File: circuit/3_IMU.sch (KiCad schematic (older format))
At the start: 23 parts

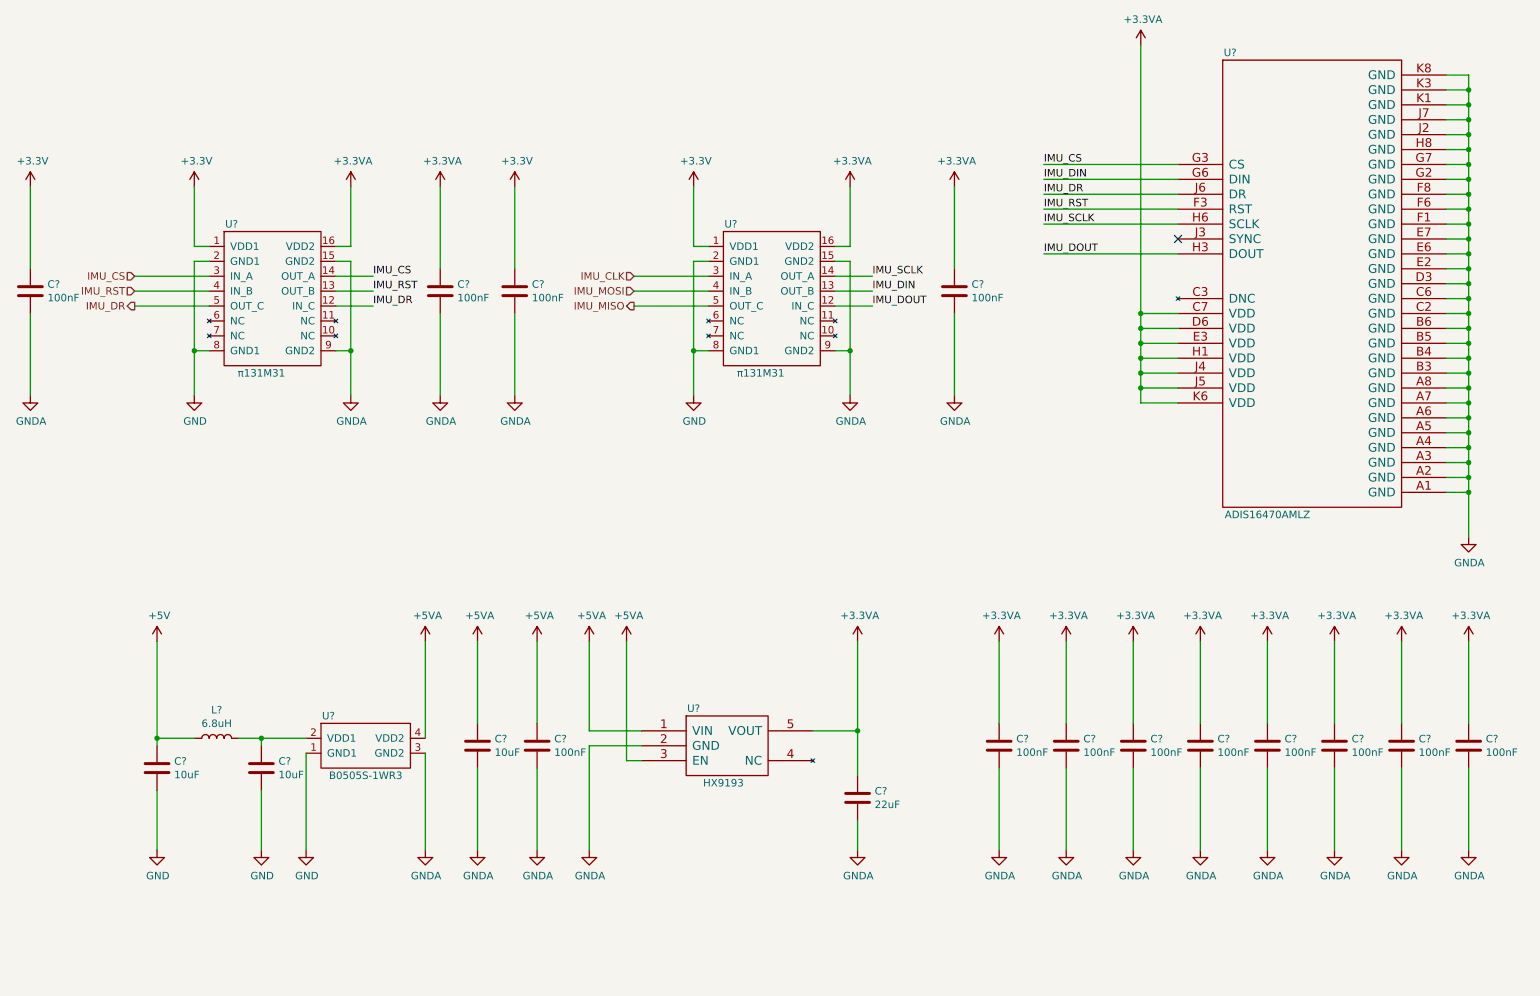
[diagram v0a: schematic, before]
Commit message: Adjust the schematic layout and add annotations to make the schematic more beautiful.
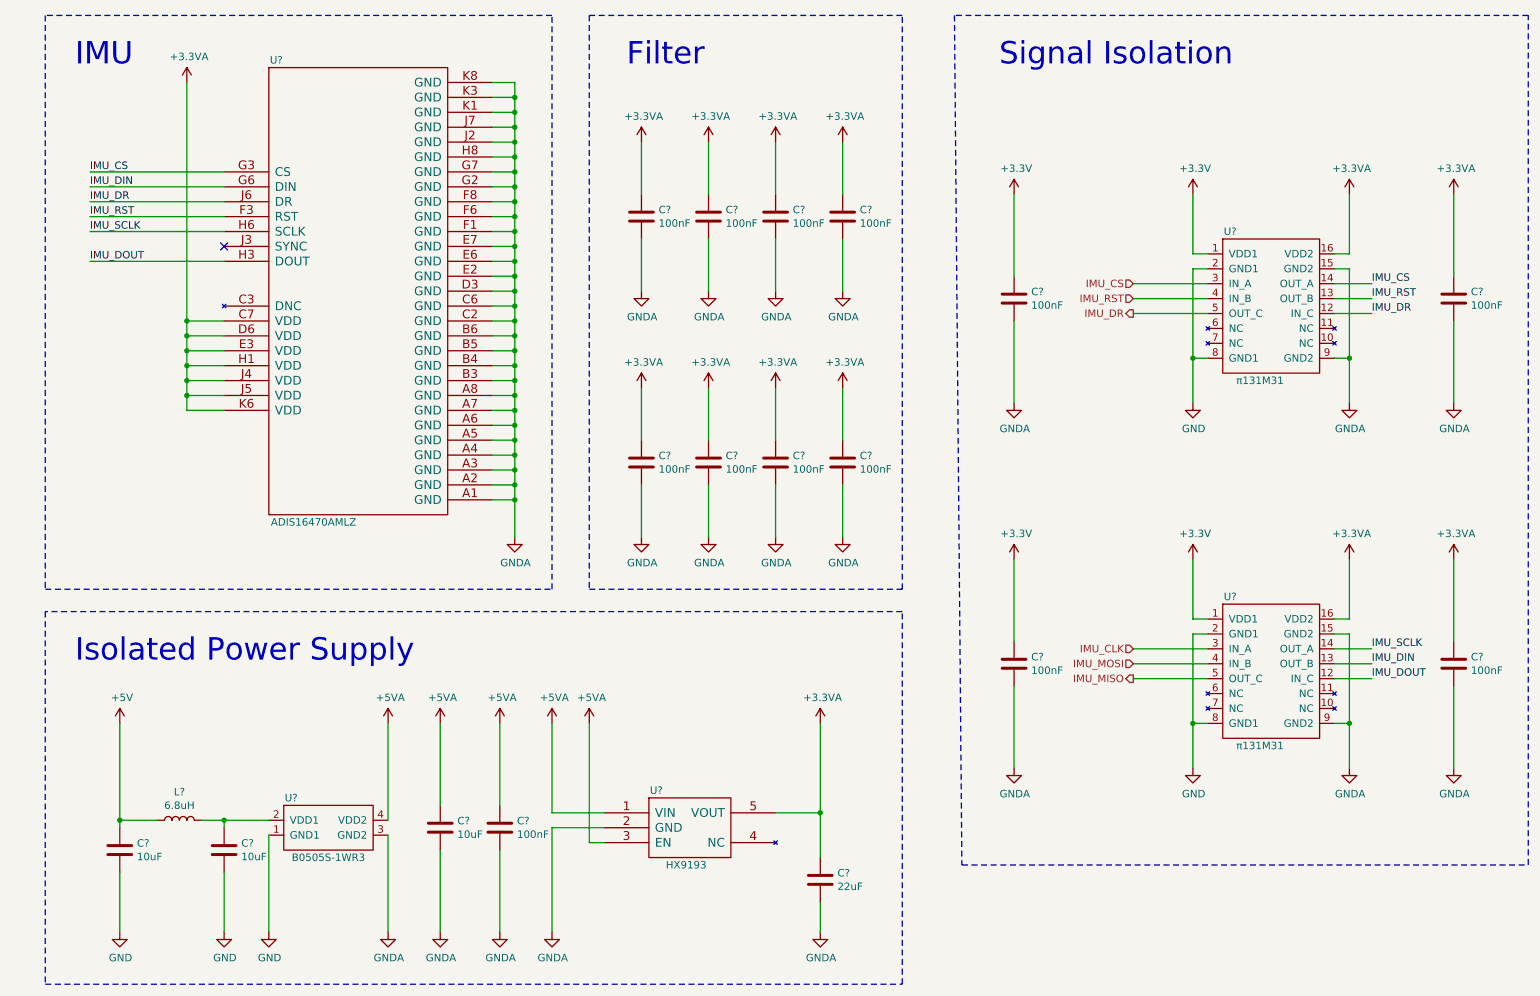
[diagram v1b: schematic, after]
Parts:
- removed C? (x11): 100nF, symbol Device:C
- removed U? (x2): π131M31, Package_SO:SOIC-16_3.9x9.9mm_P1.27mm, symbol MM32_Periph:π131M31
- added C? (x11): 100nF, symbol Device:C
- added U? (x2): π131M31, Package_SO:SOIC-16_3.9x9.9mm_P1.27mm, symbol MM32_Periph:π131M31
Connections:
- net +3.3VA: now also C?.1, C?.1, C?.1, C?.1, C?.1, C?.1, C?.1, C?.1, C?.1, U?.16 (VDD2), U?.16 (VDD2)
- net +3V3: now also C?.1, C?.1, U?.1 (VDD1), U?.1 (VDD1)
- net GND: now also U?.2 (GND1), U?.2 (GND1), U?.8 (GND1), U?.8 (GND1)
- net GNDA: now also C?.2, C?.2, C?.2, C?.2, C?.2, C?.2, C?.2, C?.2, C?.2, C?.2, C?.2, U?.15 (GND2), U?.15 (GND2), U?.9 (GND2), U?.9 (GND2)
- net IMU_CLK: now also U?.3 (IN_A)
- net IMU_CS: now also U?.14 (OUT_A), U?.3 (IN_A)
- net IMU_DIN: now also U?.13 (OUT_B)
- net IMU_DOUT: now also U?.12 (IN_C)
- net IMU_DR: now also U?.12 (IN_C), U?.5 (OUT_C)
- net IMU_MISO: now also U?.5 (OUT_C)
- net IMU_MOSI: now also U?.4 (IN_B)
- net IMU_RST: now also U?.13 (OUT_B), U?.4 (IN_B)
- net IMU_SCLK: now also U?.14 (OUT_A)
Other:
- note added: "Filter"
- note added: "IMU"
- note added: "Isolated Power Supply"
- note added: "Signal Isolation"
- moved on the sheet: C?, L?, U?
